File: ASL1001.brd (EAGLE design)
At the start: 9 x 5.1 mm, 5 parts

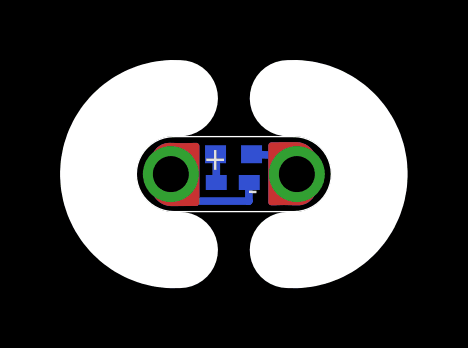
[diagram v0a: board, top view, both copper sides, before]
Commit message: Update to Rev 2
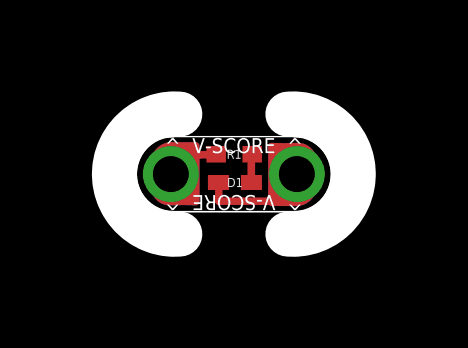
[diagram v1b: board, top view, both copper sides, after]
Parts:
- moved U$1 4.20 mm to (17.9, 20.0), flipped to the bottom
- moved U$7 4.20 mm to (22.1, 20.0), flipped to the bottom
- moved D1 0.07 mm to (20.0, 19.7), flipped to the top
- flipped R1 to the top
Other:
- board size 9 x 5.1 mm -> 8 x 4 mm
- board text added: "2"
- board text added: "^ V-SCORE ^"
- board text removed: "1"
